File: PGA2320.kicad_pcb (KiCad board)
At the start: 2 copper layers, 50 x 50 mm, 43 parts, among them J1 XH2.54-3P, J2 XH2.54-3P, J3 2P-2.54, J4 3P-2.54, P1 SDO_TO_OTHER_PGA2311, P2 CONTROLLER, Q1 BC550, Q2 BC560, U1 PGA2320

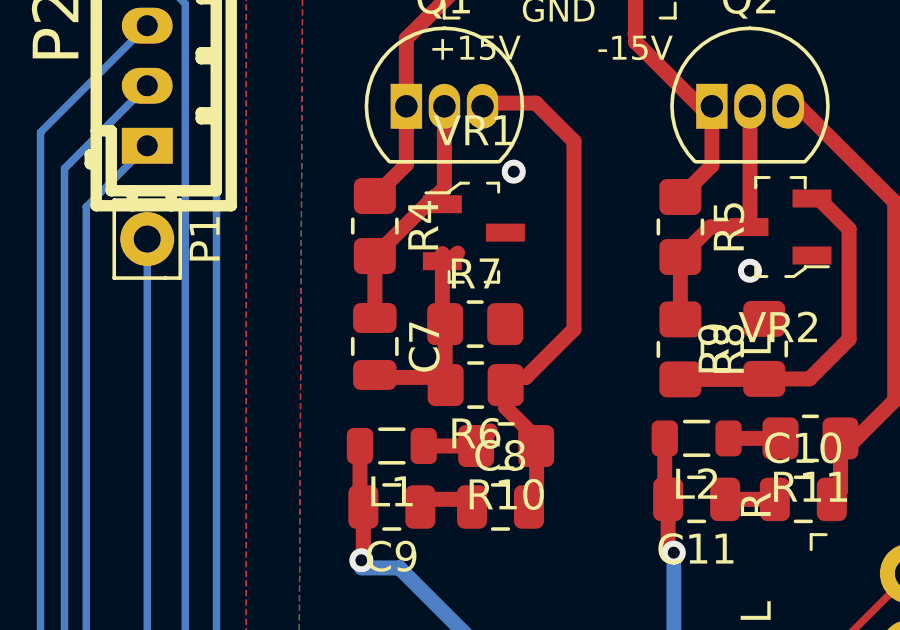
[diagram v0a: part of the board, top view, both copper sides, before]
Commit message: improvements
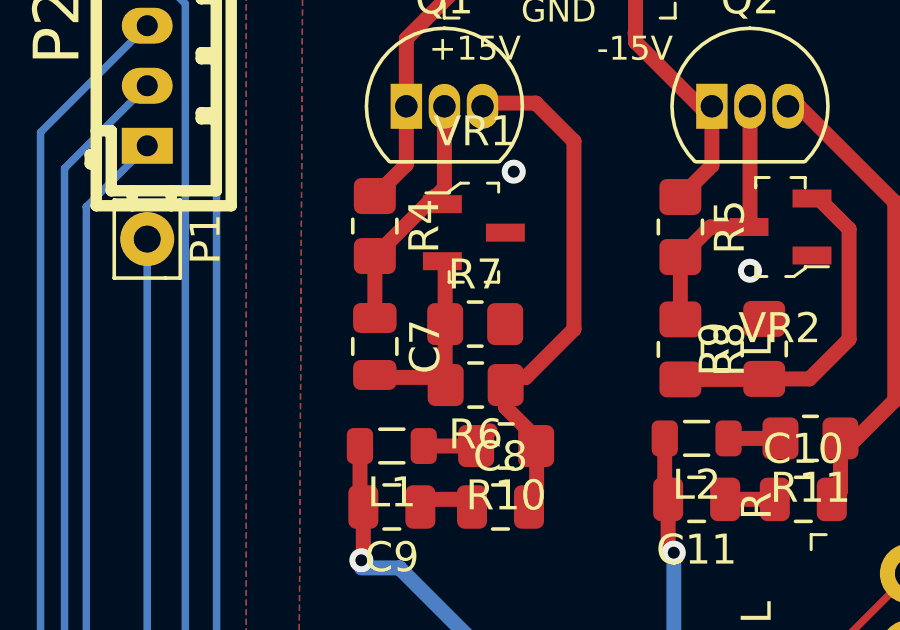
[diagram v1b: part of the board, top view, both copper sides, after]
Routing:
- net Net-(VR1-REF): track 6.88 -> 6.32 mm
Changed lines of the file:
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@@
   (segment (start 145 72.956) (end 145 75.02) (width 0.5) (layer "F.Cu") (net 19))
   (segment (start 147.32 70.684) (end 147.032 70.972) (width 0.5) (layer "F.Cu") (net 19))
-  (segment (start 147.3455 74.716) (end 147.3455 76.986) (width 0.5) (layer "F.Cu") (net 20))
-  (segment (start 147.252 72.872) (end 147.252 74.6225) (width 0.5) (layer "F.Cu") (net 20))
-  (segment (start 147.54 73.076) (end 147.76 72.856) (width 0.5) (layer "F.Cu") (net 20))
-  (segment (start 147.252 74.6225) (end 147.3455 74.716) (width 0.5) (layer "F.Cu") (net 20))
+  (segment (start 145.082 77.002) (end 145 76.92) (width 0.5) (layer "F.Cu") (net 20))
+  (segment (start 147.3455 73.2195) (end 147.3455 76.986) (width 0.5) (layer "F.Cu") (net 20))
+  (segment (start 147.252 73.126) (end 147.3455 73.2195) (width 0.5) (layer "F.Cu") (net 20))
+  (segment (start 147.3455 76.986) (end 147.3615 77.002) (width 0.5) (layer "F.Cu") (net 20))
   (segment (start 147.3615 77.002) (end 145.082 77.002) (width 0.5) (layer "F.Cu") (net 20))
-  (segment (start 145.082 77.002) (end 145 76.92) (width 0.5) (layer "F.Cu") (net 20))
-  (segment (start 147.3455 76.986) (end 147.3615 77.002) (width 0.5) (layer "F.Cu") (net 20))
   (segment (start 156.1855 71.988) (end 155.1855 72.988) (width 0.5) (layer "F.Cu") (net 21))
   (segment (start 157.5055 71.802) (end 157.6915 71.988) (width 0.5) (layer "F.Cu") (net 21))
